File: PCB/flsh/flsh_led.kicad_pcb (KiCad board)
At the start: 2 copper layers, 40 x 40 mm, 19 parts

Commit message: clean up tracks and vias
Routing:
- net Net-(LED3-A): track 10.7 -> 9.59 mm
- net Net-(LED8-A): track 16.3 -> 15.2 mm
- net Net-(LED9-A): track 14.8 -> 13.8 mm
- net Net-(LED7-A): track 13.6 -> 12.5 mm
- net Net-(LED4-A): track 10.7 -> 9.68 mm
- net Net-(LED1-A): track 15.1 -> 14.0 mm
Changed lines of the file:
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@@
-	)
-	(segment
-		(start 58 36)
-		(end 58 34.95)
-		(width 1)
-		(layer "F.Cu")
-		(net "Net-(LED9-A)")
 	)
 	(segment
@@
 	)
 	(segment
-		(start 58 41)
-		(end 58 40.975)
-		(width 1)
-		(layer "F.Cu")
-		(net "Net-(LED8-A)")
-	)
-	(segment
 		(start 58 39.95)
 		(end 56.4 38.35)
@@
 	)
 	(segment
-		(start 58 41)
-		(end 58 39.95)
-		(width 1)
-		(layer "F.Cu")
-		(net "Net-(LED8-A)")
-	)
-	(segment
 		(start 48 31)
 		(end 51.4 31)
@@
 	)
 	(segment
-		(start 53 31)
-		(end 53 32.05)
-		(width 1)
-		(layer "F.Cu")
-		(net "Net-(LED3-A)")
-	)
-	(segment
 		(start 54.52 31)
 		(end 54.52 27.545)
@@
 	)
 	(segment
-		(start 54.52 27.545)
-		(end 54.475 27.5)
-		(width 1)
-		(layer "F.Cu")
-		(net "Net-(LED3-A)")
-	)
-	(segment
 		(start 54.475 44.5)
 		(end 56.525 44.5)
@@
 	)
 	(segment
-		(start 48 36)
-		(end 48 34.95)
-		(width 1)
-		(layer "F.Cu")
-		(net "Net-(LED1-A)")
-	)
-	(segment
 		(start 46.5 27.5)
 		(end 46.4 27.6)
@@
 	)
 	(segment
-		(start 48 41)
-		(end 48 39.95)
-		(width 1)
-		(layer "F.Cu")
-		(net "Net-(LED7-A)")
-	)
-	(segment
 		(start 46.4 42)
 		(end 46.4 41)
@@
 		(width 1)
 		(layer "F.Cu")
-		(net "Net-(LED4-A)")
-	)
-	(segment
-		(start 53 37.05)
-		(end 53 36)
-		(width 1)
-		(layer "F.Cu")

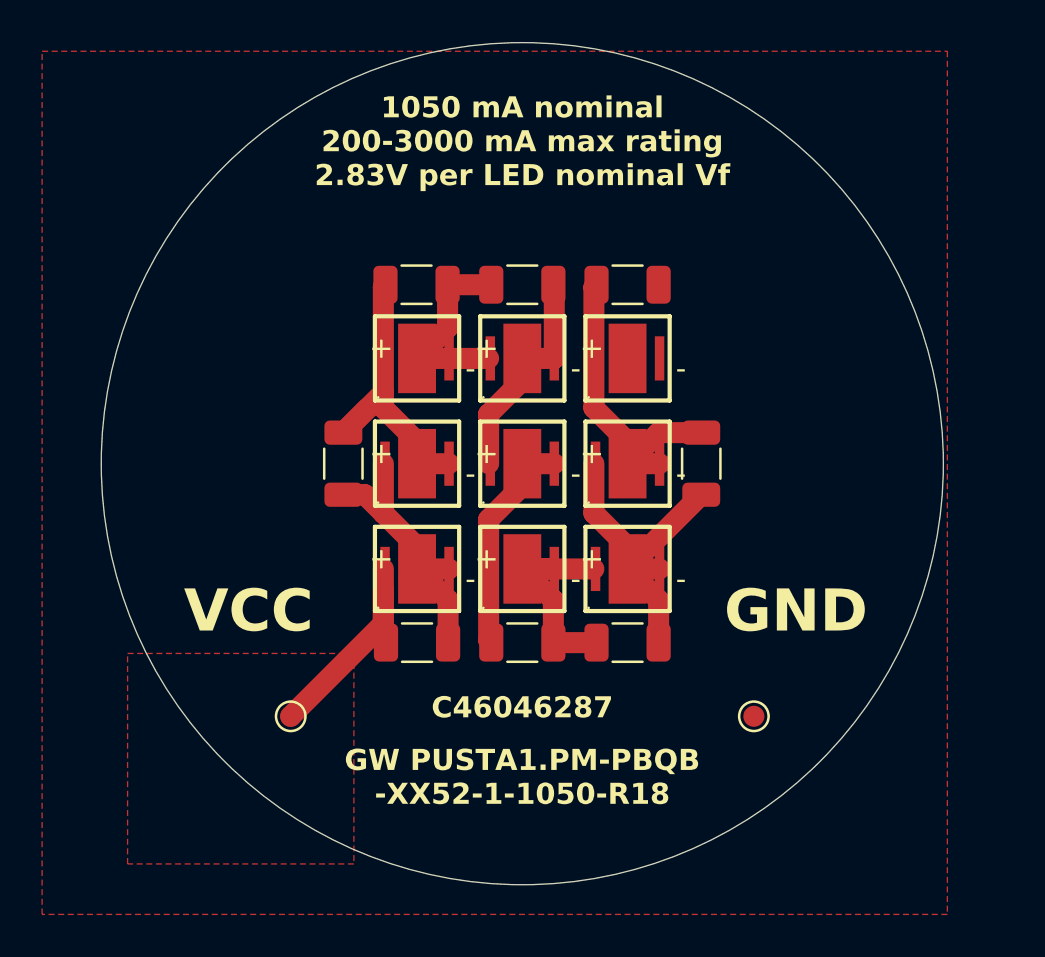
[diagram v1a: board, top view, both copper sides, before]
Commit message: l
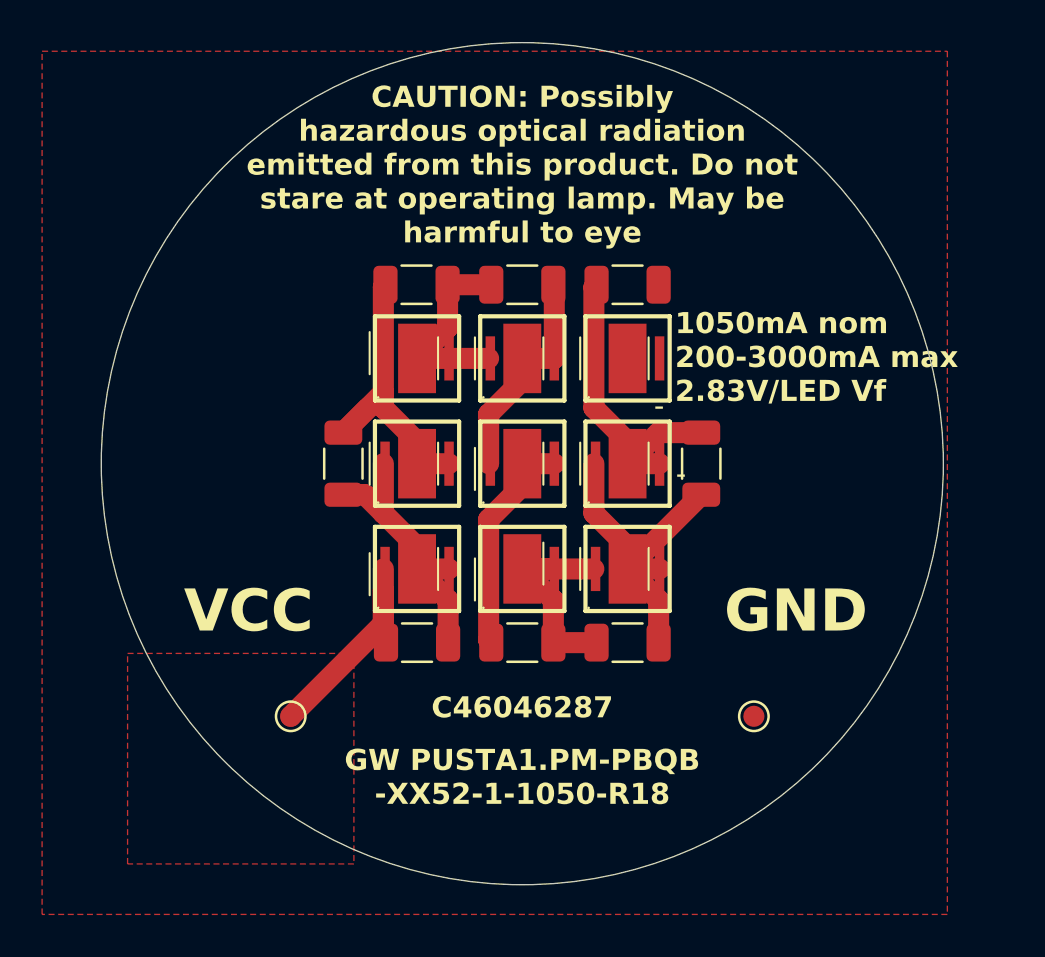
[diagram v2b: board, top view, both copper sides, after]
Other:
- board text added: "1050mA nom 200-3000mA max 2.83V/LED Vf"
- board text added: "CAUTION: Possibly hazardous optical radiation emitted from this product. Do not stare at operating lamp. May be harmful to eye"
- board text removed: "1050 mA nominal 200-3000 mA max rating 2.83V per LED nominal Vf"
